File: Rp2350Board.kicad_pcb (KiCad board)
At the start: 4 copper layers, 50 x 25 mm, 42 parts, among them J1 Conn_01x04, J2 Conn_01x02, J3 Conn_01x02, J4 Conn_01x06, J5 Conn_01x06, SW1 SW_Push, SW2 SW_Push, U1 RP2350A-QFN60, U2 LD1117V33, U3 W25Q128JVS, U5 SN65HVD232, Y1 ABM8-272-T3

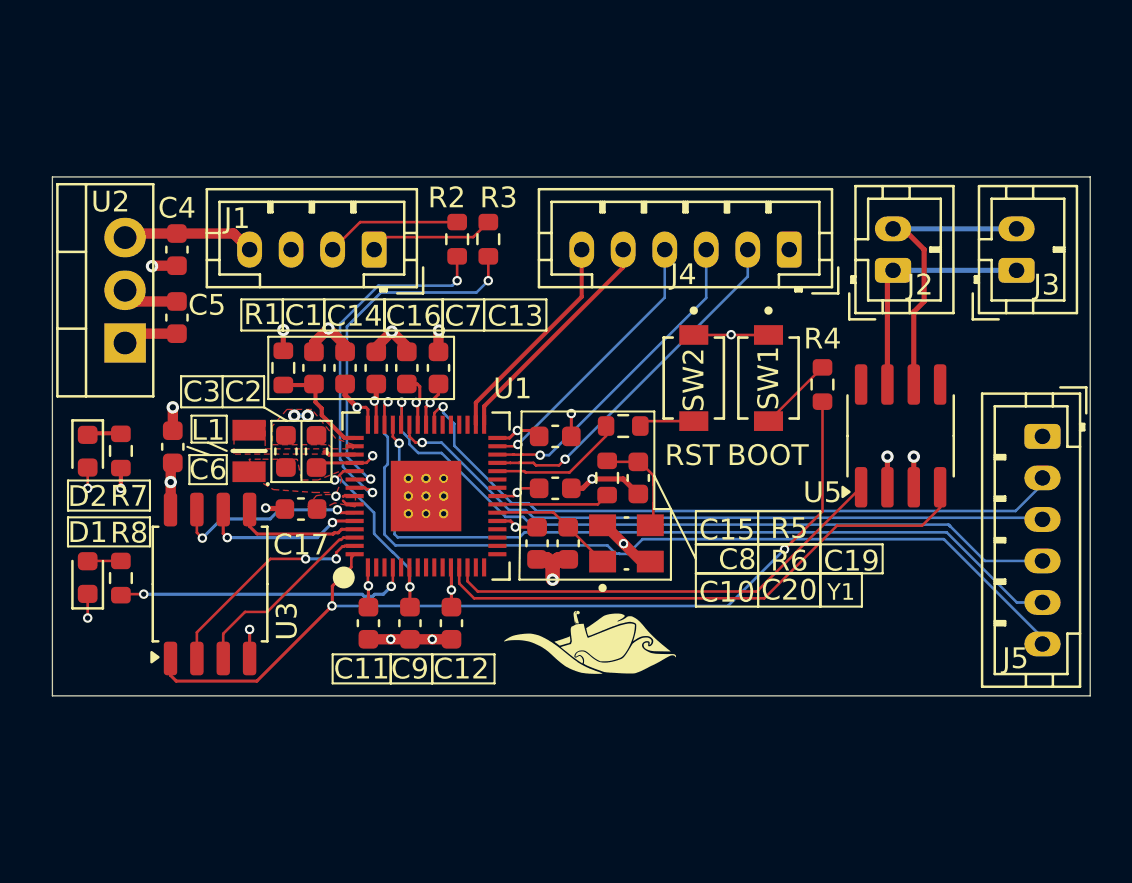
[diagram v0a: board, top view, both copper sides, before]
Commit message: First draft of v2 board
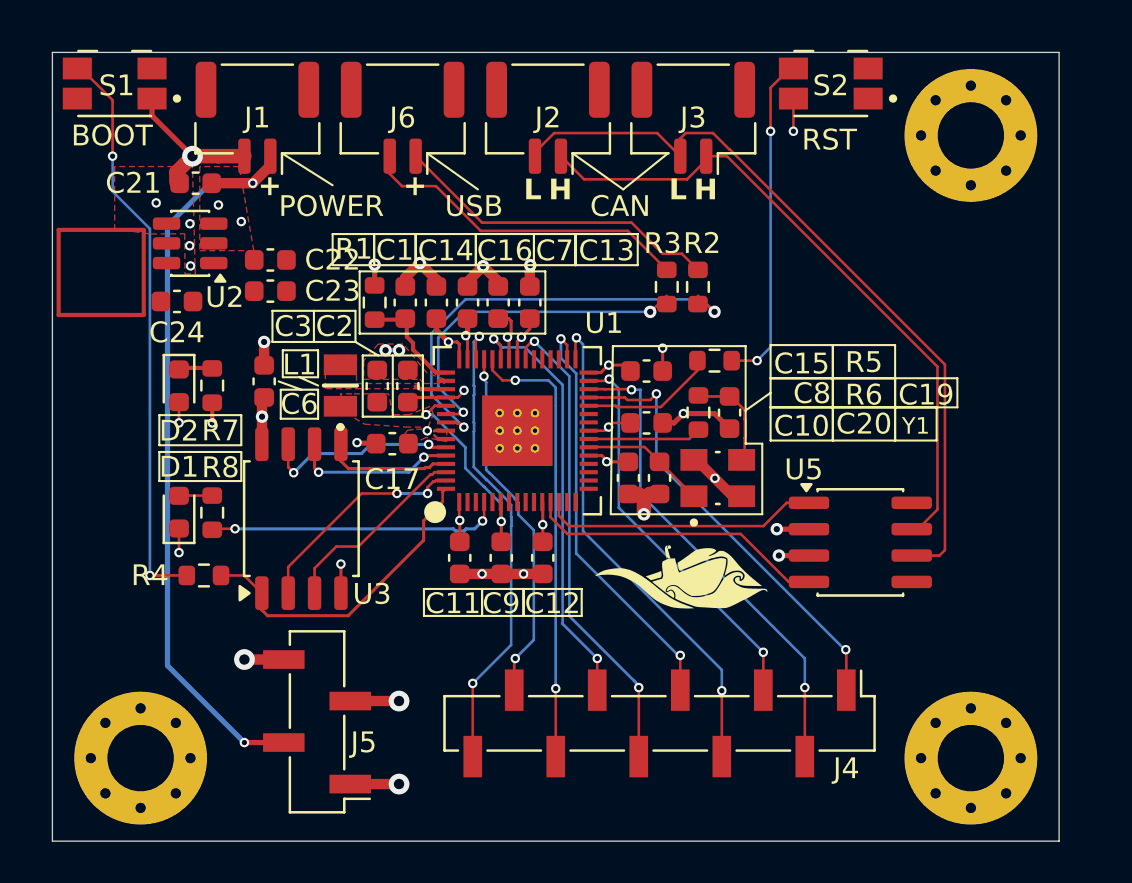
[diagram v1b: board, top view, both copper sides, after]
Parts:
- removed C4: 100n, Capacitor_SMD:C_0603_1608Metric
- removed C5: 10u, Capacitor_SMD:C_0603_1608Metric
- removed SW1, SW2: SW_Push, ProjectLibrary:SW_TL1015AF160QG
- added C21: 10u, Capacitor_SMD:C_0603_1608Metric, F.Cu at (122.4, 82.3)
- added C22: 22u, Capacitor_SMD:C_0603_1608Metric, F.Cu at (126.0, 86.0)
- added C23: 22u, Capacitor_SMD:C_0603_1608Metric, F.Cu at (126.0, 87.5)
- added C24: 100n, Capacitor_SMD:C_0603_1608Metric, F.Cu at (121.5, 88.0)
- added J6: Conn_01x02, Connector_JST:JST_GH_SM02B-GHS-TB_1x02-1MP_P1.25mm_Horizontal, F.Cu at (132.4, 79.2)
- added REF**: MountingHole_3.2mm_M3_Pad_Via, MountingHole:MountingHole_3.2mm_M3_Pad_Via, F.Cu at (159.8, 80.0)
- added REF**: MountingHole_3.2mm_M3_Pad_Via, MountingHole:MountingHole_3.2mm_M3_Pad_Via, F.Cu at (119.8, 110.0)
- added REF**: MountingHole_3.2mm_M3_Pad_Via, MountingHole:MountingHole_3.2mm_M3_Pad_Via, F.Cu at (159.8, 110.0)
- added S1: EVQ-P7A01P, ProjectLibrary:SW_EVQ-P7A01P, F.Cu at (118.5, 77.5)
- added S2: EVQ-P7A01P, ProjectLibrary:SW_EVQ-P7A01P, F.Cu at (153.0, 77.5)
- J1: value Conn_01x04 -> Conn_01x02; footprint Connector_JST:JST_PH_B4B-PH-K_1x04_P2.00mm_Vertical -> Connector_JST:JST_GH_SM02B-GHS-TB_1x02-1MP_P1.25mm_Horizontal
- J2, J3: footprint Connector_JST:JST_PH_B2B-PH-K_1x02_P2.00mm_Vertical -> Connector_JST:JST_GH_SM02B-GHS-TB_1x02-1MP_P1.25mm_Horizontal
- J4: value Conn_01x06 -> Conn_01x10; footprint Connector_JST:JST_PH_B6B-PH-K_1x06_P2.00mm_Vertical -> Connector_PinSocket_2.00mm:PinSocket_1x10_P2.00mm_Vertical_SMD_Pin1Left
- J5: value Conn_01x06 -> Conn_01x04; footprint Connector_JST:JST_PH_B6B-PH-K_1x06_P2.00mm_Vertical -> Connector_PinSocket_2.00mm:PinSocket_1x04_P2.00mm_Vertical_SMD_Pin1Left
- U2: value LD1117V33 -> AP63203WU; footprint Package_TO_SOT_THT:TO-220-3_Vertical -> Package_TO_SOT_SMD:TSOT-23-6
- moved J5 37.6 mm to (128.2, 108.2), turned to 180 degrees
- moved R4 31.2 mm to (122.8, 101.2), turned to 180 degrees
- moved J4 23.7 mm to (144.8, 108.3), turned to -90 degrees
- moved J2 18.2 mm to (139.4, 79.2), turned to 180 degrees
- moved J3 17.2 mm to (146.4, 79.2), turned to 180 degrees
- moved R2 11.8 mm to (146.6, 87.3)
- moved R3 8.90 mm to (145.1, 87.3)
- moved J1 8.48 mm to (125.4, 79.2)
- moved U2 5.73 mm to (122.1, 85.2), turned to 180 degrees
- moved U5 5.48 mm to (154.4, 99.6), turned to 0 degrees
- moved C1 5.41 mm to (132.5, 88.0)
- moved C10 5.41 mm to (143.2, 96.5)
- moved C11 5.41 mm to (135.1, 100.3)
- moved C12 5.41 mm to (139.1, 100.3)
- moved C13 5.41 mm to (138.5, 88.0)
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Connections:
- J1 pad 1: USB D- -> VBUS
- J1 pad 2: USB D+ -> GND
- J4 pad 1: GND -> Net-(J4-Pin_1)
- J5 pad 2: Net-(J5-Pin_2) -> VBUS
- J5 pad 3: Net-(J5-Pin_3) -> +3V3
- J5 pad 4: Net-(J5-Pin_4) -> GND
- R5 pad 1: Net-(R5-Pad1) -> /RST
- U1 pad 27: Net-(J4-Pin_2) -> Net-(J4-Pin_1)
- U1 pad 28: Net-(J4-Pin_3) -> Net-(J4-Pin_2)
- U1 pad 29: Net-(J4-Pin_4) -> Net-(J4-Pin_3)
- U1 pad 31: Net-(J4-Pin_5) -> Net-(J4-Pin_4)
- U1 pad 32: Net-(J4-Pin_6) -> Net-(J4-Pin_5)
- U1 pad 37: Net-(J5-Pin_2) -> Net-(J4-Pin_6)
- U1 pad 40: Net-(J5-Pin_3) -> Net-(J4-Pin_7)
- U1 pad 41: Net-(J5-Pin_4) -> Net-(J4-Pin_8)
- U1 pad 42: Net-(J5-Pin_5) -> Net-(J4-Pin_9)
- U1 pad 43: Net-(J5-Pin_6) -> Net-(J4-Pin_10)
- U2 pad 1: GND -> +3V3
- U2 pad 2: +3V3 -> VBUS
- U2 pad 3: +5V -> VBUS
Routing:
- net Net-(J5-Pin_6): track 42.4 -> 0.00 mm, vias 1 -> 0
- net Net-(J5-Pin_5): track 38.8 -> 0.00 mm, vias 1 -> 0
- net VBUS: track 0.00 -> 37.1 mm, vias 0 -> 4
- net Net-(J5-Pin_4): track 36.8 -> 0.00 mm, vias 1 -> 0
- net Net-(J5-Pin_2): track 33.8 -> 0.00 mm, vias 1 -> 0
- net Net-(J5-Pin_3): track 33.5 -> 0.00 mm, vias 1 -> 0
- net FLASH_SS: track 44.0 -> 15.5 mm, vias 2 -> 0
- net USB_BOOT: track 3.67 -> 27.8 mm, vias 0 -> 2
- net Net-(J4-Pin_10): track 0.00 -> 23.2 mm, vias 0 -> 2
- net CANL-: track 14.6 -> 37.0 mm
- net Net-(J4-Pin_8): track 0.00 -> 21.7 mm, vias 0 -> 2
- net Net-(J4-Pin_1): track 0.00 -> 21.5 mm, vias 0 -> 2
- net Net-(J4-Pin_7): track 0.00 -> 20.9 mm, vias 0 -> 2
- net CANH+: track 11.6 -> 31.9 mm
- net Net-(J4-Pin_9): track 0.00 -> 17.3 mm, vias 0 -> 2
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- added copper zone on F.Cu, net VBUS
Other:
- board size 50 x 25 mm -> 48.5 x 38 mm
- board text added: "+"
- board text added: "CAN"
- board text added: "H"
- board text added: "L"
- board text added: "POWER"
- board text added: "USB"
- board text added: "WSU RoboSub RP2350 PCB Designed Spring2026 by Daniel Bereza"
- board text removed: "WSU RoboSub RP2350 PCB Designed Fall2025 by Daniel Bereza"

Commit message: Small edits to first draft of v2
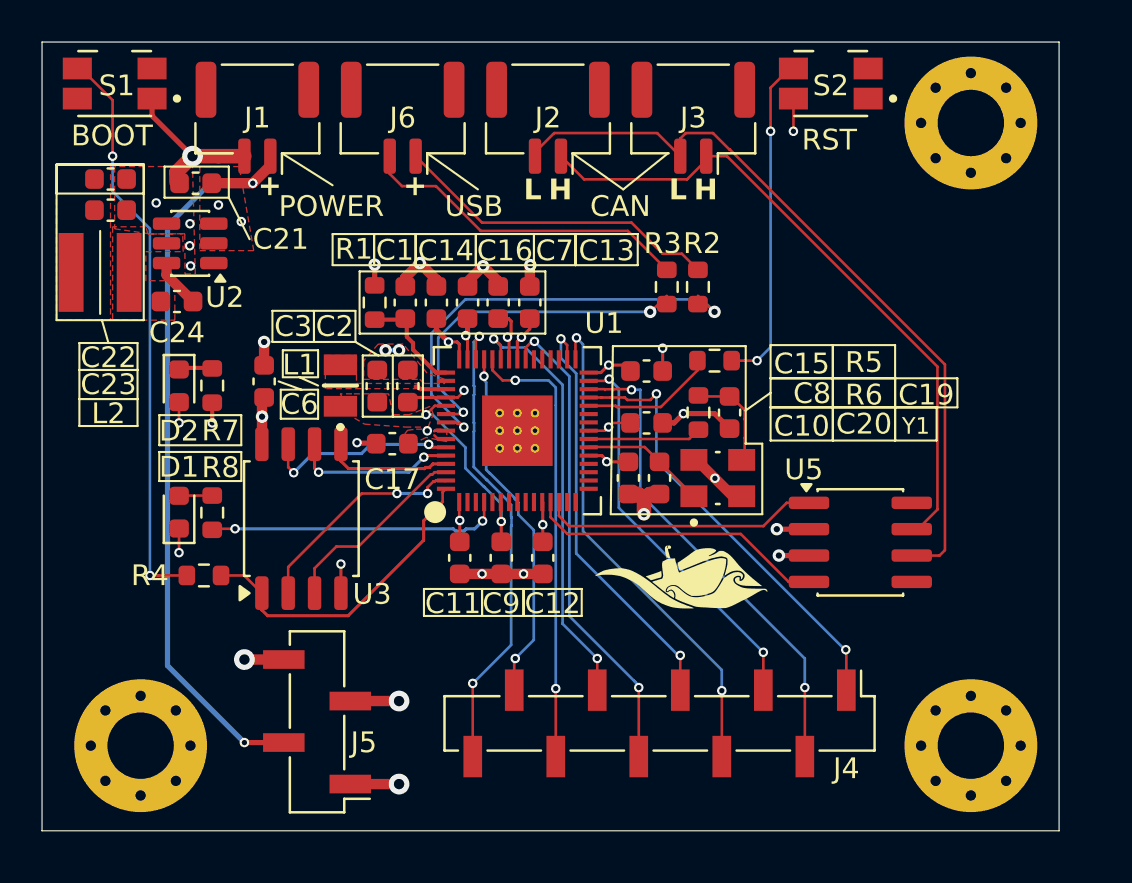
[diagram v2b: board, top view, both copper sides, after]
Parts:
- added L2: L, ProjectLibrary:PA5430, F.Cu at (117.8, 86.6)
- moved C22 8.63 mm to (118.3, 82.1)
- moved C23 8.63 mm to (118.3, 83.6)
- moved REF** 0.60 mm to (159.8, 79.4)
- moved REF** 0.60 mm to (119.8, 109.4)
- moved REF** 0.60 mm to (159.8, 109.4)
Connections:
- net Net-(U2-SW) renamed /REG_SW
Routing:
- net Net-(U2-BST): track 0.00 -> 2.38 mm
- added copper zone on F.Cu, net /REG_SW
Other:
- board size 48.5 x 38 mm -> 49 x 38 mm
